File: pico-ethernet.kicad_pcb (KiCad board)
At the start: 2 copper layers, 51 x 22 mm, 29 parts, among them J1 Conn_01x20_Pin, J2 Conn_01x02, J3 VR05S05, J4 SI-52003-F, J5 Conn_01x02, J6 Conn_01x02_Pin, U1 ENC28J60x-SS, Y1 25MHz

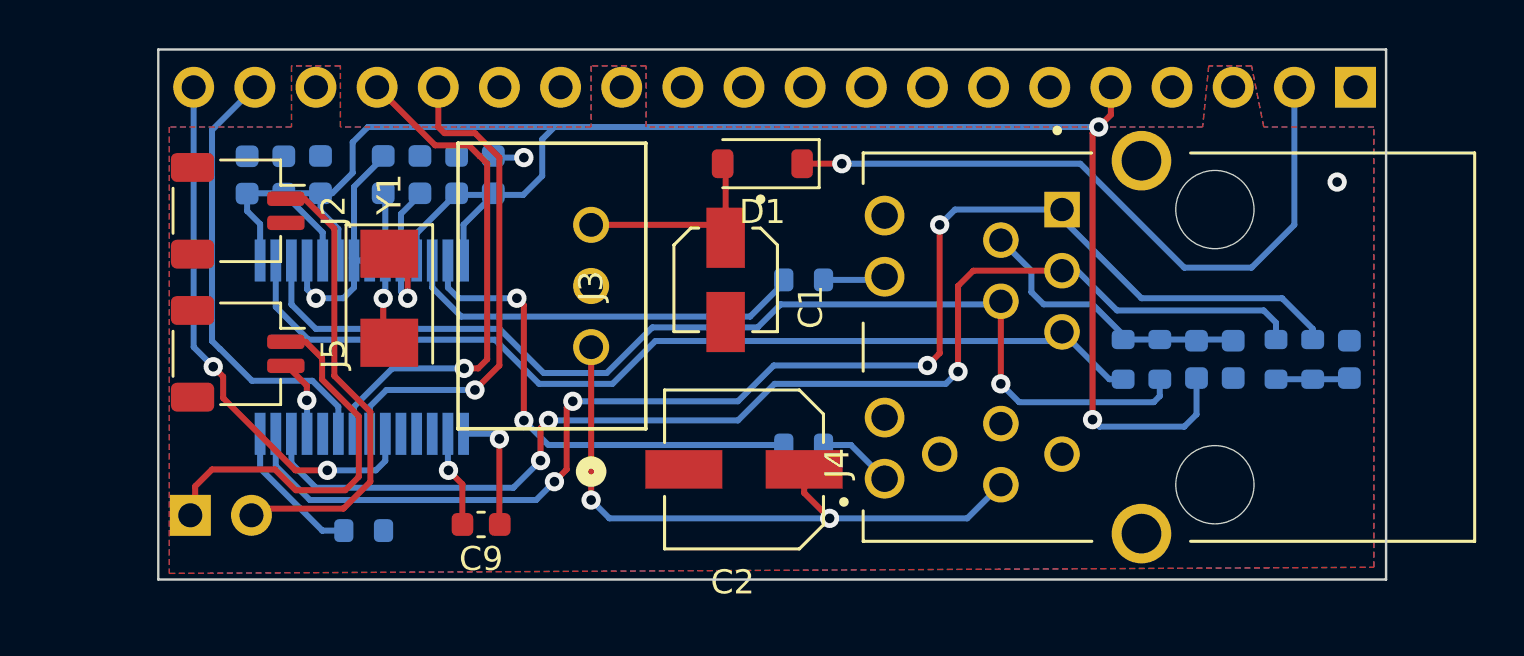
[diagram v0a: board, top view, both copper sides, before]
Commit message: redux 1?
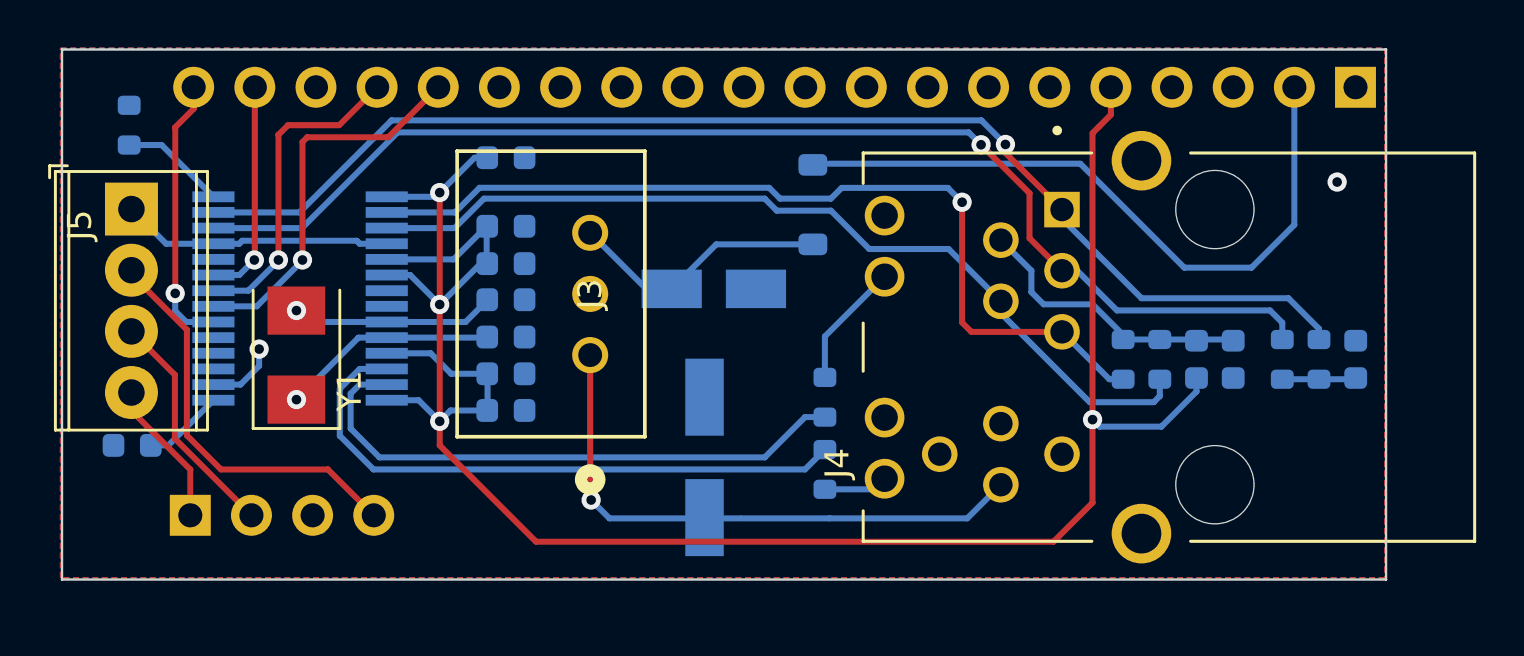
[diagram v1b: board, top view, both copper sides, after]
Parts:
- removed the J2 at (146.6, 116.3)
- C1, C2, C9, D1: moved to B.Cu
- J2: renamed from J6; footprint Connector_PinSocket_2.54mm:PinSocket_1x02_P2.54mm_Vertical -> Connector_PinSocket_2.54mm:PinSocket_1x04_P2.54mm_Vertical
- J5: footprint Connector_JST:JST_SH_SM02B-SRSS-TB_1x02-1MP_P1.00mm_Horizontal -> TerminalBlock_Phoenix:TerminalBlock_Phoenix_MPT-0,5-4-2.54_1x04_P2.54mm_Horizontal
- moved R1 19.5 mm to (142.1, 112.7), turned to 90 degrees
- moved C9 14.9 mm to (142.2, 126.0)
- moved C3 12.5 mm to (157.8, 124.5), turned to 0 degrees
- moved C10 12.4 mm to (157.8, 123.0), turned to 0 degrees
- moved C11 11.4 mm to (157.8, 118.5), turned to 0 degrees
- moved C6 7.63 mm to (157.8, 121.5), turned to 180 degrees
- moved J5 7.46 mm to (142.2, 116.2)
- moved C5 7.28 mm to (157.8, 120.0), turned to 180 degrees
- moved R6 4.95 mm to (171.0, 124.0), turned to 90 degrees
- moved Y1 4.52 mm to (149.1, 122.2), turned to 90 degrees
- moved U1 3.26 mm to (149.2, 119.9), turned to 0 degrees
- moved D1 2.70 mm to (170.5, 116.0), turned to -90 degrees
- moved C4 2.21 mm to (157.8, 116.9), turned to 0 degrees
- moved C12 2.17 mm to (157.8, 114.0), turned to 180 degrees
- moved C2 1.71 mm to (166.0, 126.5), turned to 90 degrees
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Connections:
- J2 pad 1: Net-(J5-Pin_1) -> Net-(J2-Pin_1)
- J2 pad 2: Net-(J2-Pin_1) -> Net-(J2-Pin_2)
- J5 pad 1: Net-(J5-Pin_1) -> GND
- J5 pad 2: GND -> Net-(J2-Pin_4)
- R6 pad 1: Net-(U1-LEDB) -> Net-(U1-LEDA)
- R7 pad 1: Net-(U1-LEDA) -> Net-(U1-LEDB)
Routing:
- net Net-(J2-Pin_4): track 0.00 -> 17.0 mm
- net Net-(J5-Pin_1): track 15.9 -> 0.00 mm
- net Net-(J2-Pin_1): track 18.9 -> 6.11 mm
- net Net-(J1-Pin_20): track 22.7 -> 11.4 mm, vias 2 -> 1
- net +3.3V: track 80.0 -> 90.5 mm, vias 2 -> 4
- net Net-(J2-Pin_2): track 0.00 -> 9.70 mm
- net Net-(J1-Pin_19): track 18.8 -> 9.14 mm, vias 0 -> 1
- net Net-(U1-LEDB): track 16.9 -> 25.3 mm
- net Net-(J1-Pin_17): track 21.5 -> 13.4 mm
- net Net-(J4-RD+): track 44.9 -> 37.3 mm, vias 1 -> 0
- net Net-(J4-TD+): track 57.3 -> 52.0 mm, vias 4 -> 1
- net Net-(J1-Pin_16): track 20.6 -> 16.0 mm
- net GND: track 18.7 -> 14.2 mm, vias 5 -> 2
- net Net-(U1-LEDA): track 20.6 -> 24.2 mm, vias 2 -> 0
- net +24V: track 26.7 -> 23.9 mm, vias 2 -> 1
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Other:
- board size 51 x 22 mm -> 55 x 22 mm
